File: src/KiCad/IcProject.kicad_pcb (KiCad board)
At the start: 2 copper layers, 59.5 x 115.7 mm, 34 parts, among them J1 Screw_Terminal_01x02, U1 LM556, U2 4017, U3 4017, U4 4020, U5 4017

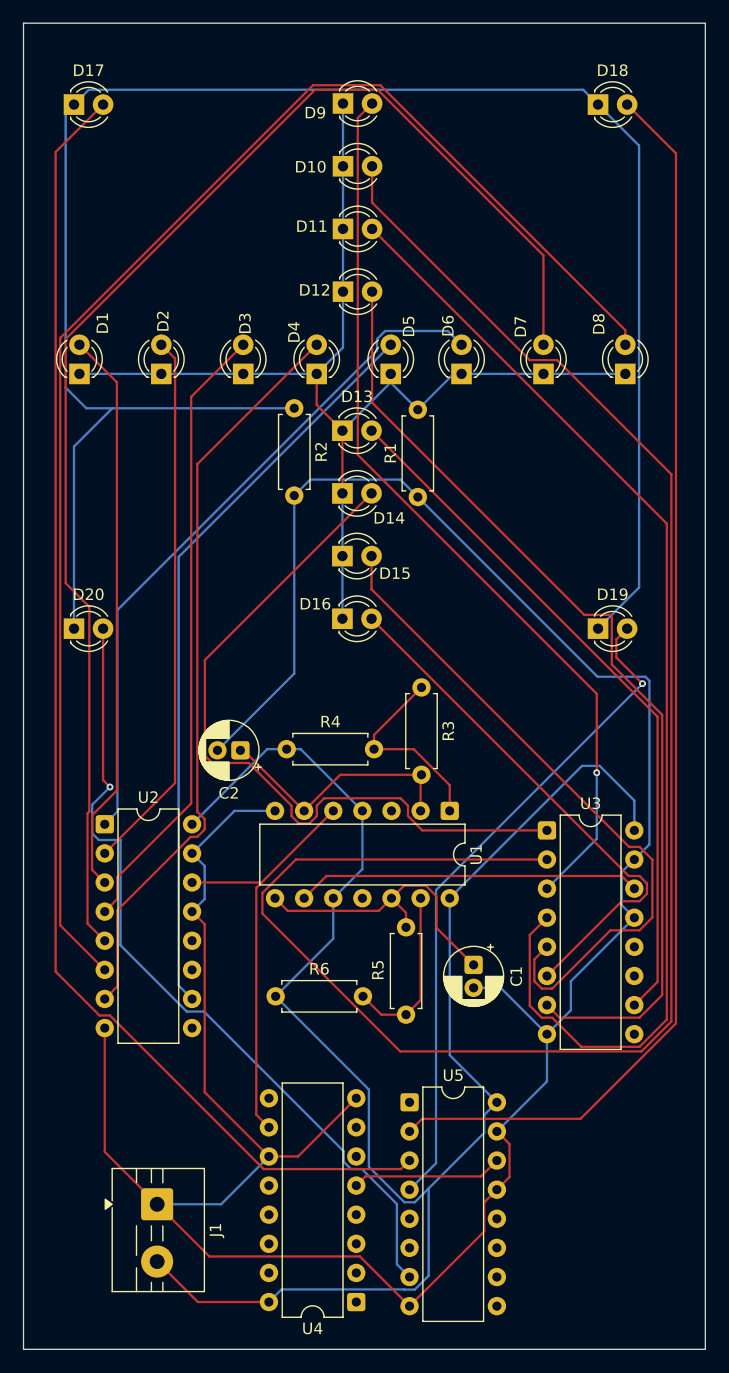
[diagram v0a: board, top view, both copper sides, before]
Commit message: updated the layout
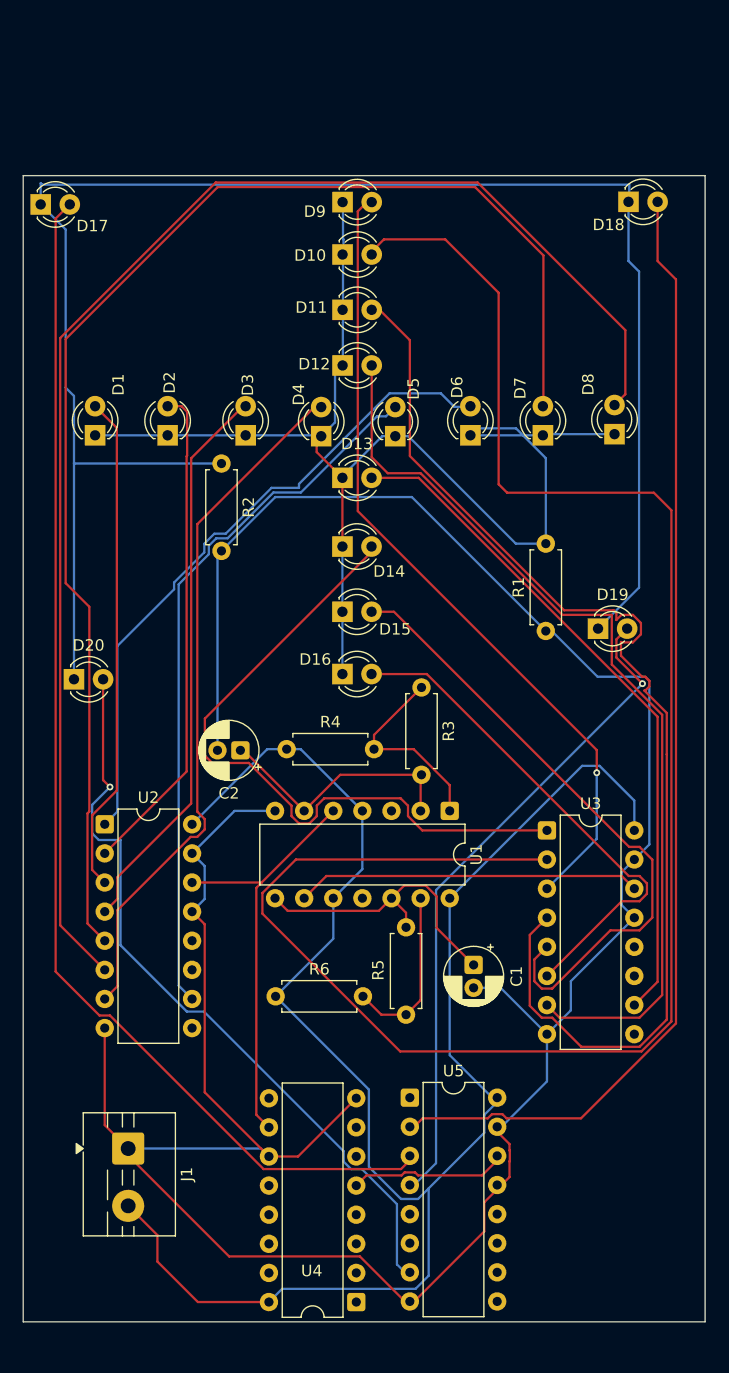
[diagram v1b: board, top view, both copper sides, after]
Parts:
- moved R1 16.2 mm to (194.4, 91.3)
- moved D17 9.18 mm to (150.3, 54.1)
- moved D18 8.89 mm to (201.6, 53.9)
- moved D9 8.60 mm to (176.7, 53.9)
- moved R2 7.98 mm to (166.1, 76.7)
- moved D10 7.70 mm to (176.7, 58.5)
- moved D11 7.06 mm to (176.7, 63.3)
- moved D12 6.44 mm to (176.7, 68.2)
- moved D1 5.53 mm to (155.1, 74.3)
- moved J1 5.48 mm to (158.0, 136.5)
- moved D4 5.45 mm to (174.8, 74.3)
- moved D5 5.45 mm to (181.3, 74.3)
- moved D6 5.41 mm to (187.8, 74.3)
- moved D2 5.39 mm to (161.4, 74.3)
- moved D3 5.36 mm to (168.2, 74.3)
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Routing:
- net Net-(D1-K): track 97.7 -> 114.2 mm
- net Net-(D17-K): track 161.8 -> 149.4 mm
- net Net-(D17-A): track 115.7 -> 105.8 mm
- net Net-(D18-A): track 109.1 -> 99.8 mm
- net Net-(D9-A): track 79.4 -> 71.1 mm
- net Net-(D1-A): track 49.6 -> 43.7 mm
- net VCC: track 152.3 -> 158.0 mm
- net Net-(D3-A): track 54.5 -> 49.4 mm
- net Net-(D4-A): track 65.6 -> 60.7 mm
- net Net-(D14-A): track 64.9 -> 60.2 mm
- net Net-(D20-A): track 71.5 -> 67.1 mm
- net Net-(D10-A): track 156.4 -> 160.6 mm
- net Net-(D2-A): track 47.4 -> 43.4 mm
- net Net-(D15-A): track 58.8 -> 55.1 mm
- net Net-(D12-A): track 84.6 -> 81.0 mm
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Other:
- board size 59.5 x 115.7 mm -> 59.5 x 100 mm
